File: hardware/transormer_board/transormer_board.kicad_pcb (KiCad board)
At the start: 2 copper layers, 25 x 45 mm, 8 parts, among them J1 orange, J2 black, J3 PE, J4 Conn_02x04_Top_Bottom, J5 red, J6 grey

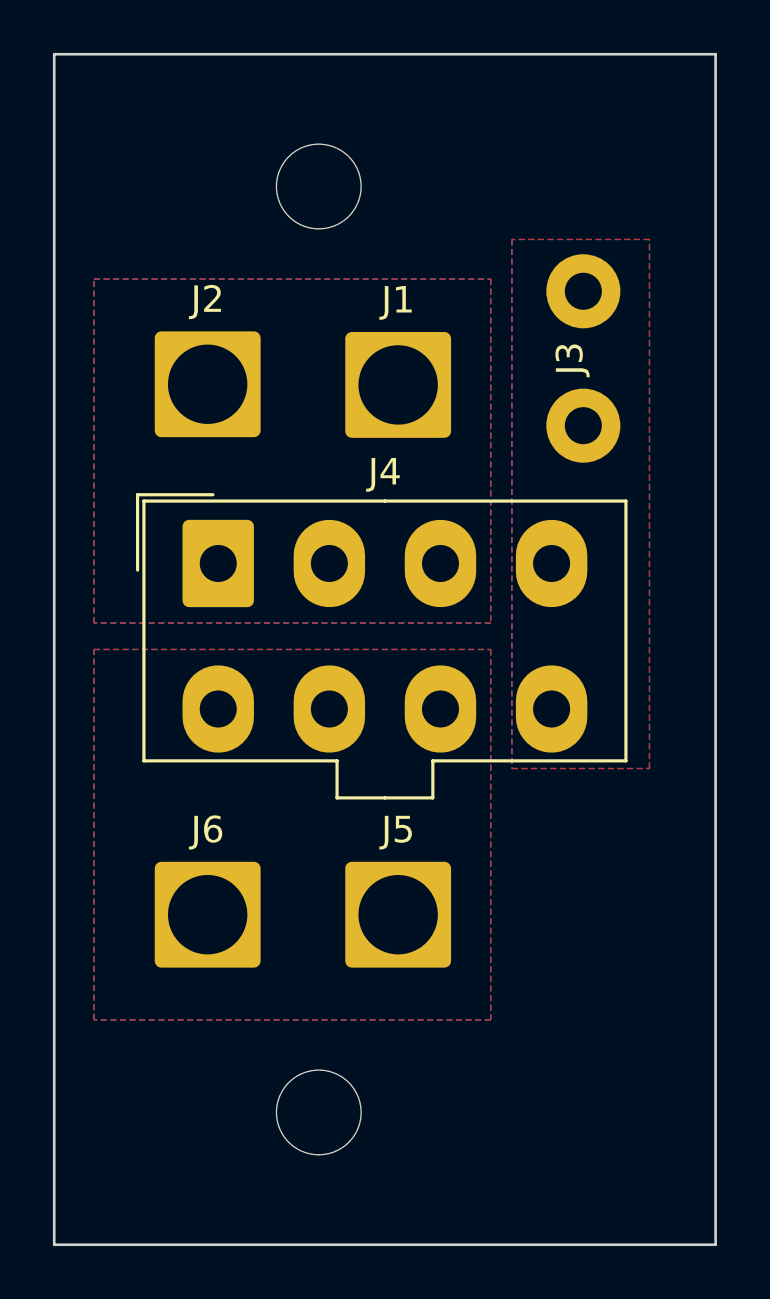
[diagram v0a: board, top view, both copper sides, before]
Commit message: update some shit
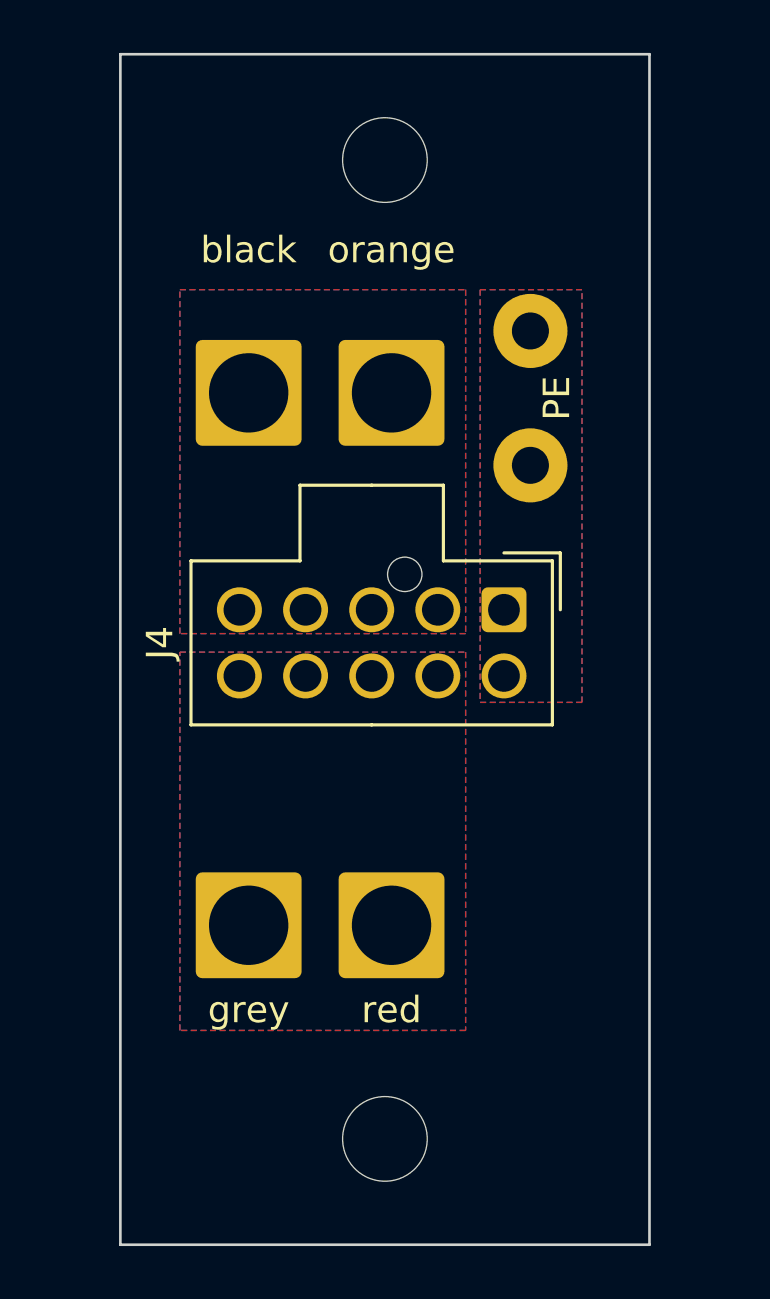
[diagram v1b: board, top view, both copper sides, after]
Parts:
- removed the REF** at (160.0, 121.0)
- removed the REF** at (160.0, 86.0)
- added REF**: MountingHole_3.2mm_M3, MountingHole:MountingHole_3.2mm_M3, F.Cu at (162.5, 122.0)
- added REF**: MountingHole_3.2mm_M3, MountingHole:MountingHole_3.2mm_M3, F.Cu at (162.5, 85.0)
- J4: footprint Connector_Molex:Molex_Mini-Fit_Jr_5566-08A_2x04_P4.20mm_Vertical -> Connector_Molex:Molex_Nano-Fit_105310-xx10_2x05_P2.50mm_Vertical
- moved J4 10.9 mm to (167.0, 102.0), turned to -90 degrees
- moved J3 2.50 mm to (168.0, 94.0)
- moved J6 1.60 mm to (157.3, 113.9)
- moved J2 1.58 mm to (157.3, 93.8)
- moved J5 0.47 mm to (162.8, 113.9)
- moved J1 0.39 mm to (162.8, 93.8)
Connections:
- J4 pad 1: Net-(J1-Pin_1) -> Net-(J3-Pin_1)
- J4 pad 4: Net-(J3-Pin_1) -> Net-(J1-Pin_1)
- J4 pad 5: Net-(J4-Pin_5) -> Net-(J1-Pin_1)
- J4 pad 6: Net-(J4-Pin_5) -> Net-(J3-Pin_1)
- J4 pad 7: Net-(J4-Pin_5) -> Net-(J4-Pin_10)
- J4 pad 8: Net-(J3-Pin_1) -> Net-(J4-Pin_10)
- J5 pad 1: Net-(J4-Pin_5) -> Net-(J4-Pin_10)
- J6 pad 1: Net-(J4-Pin_5) -> Net-(J4-Pin_10)
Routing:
- added copper zone on B.Cu, net Net-(J4-Pin_10)
- added copper zone on F.Cu, net Net-(J4-Pin_10)
- removed copper zone on B.Cu, net Net-(J4-Pin_5)
- removed copper zone on F.Cu, net Net-(J4-Pin_5)
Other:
- board size 25 x 45 mm -> 20 x 45 mm

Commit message: save work
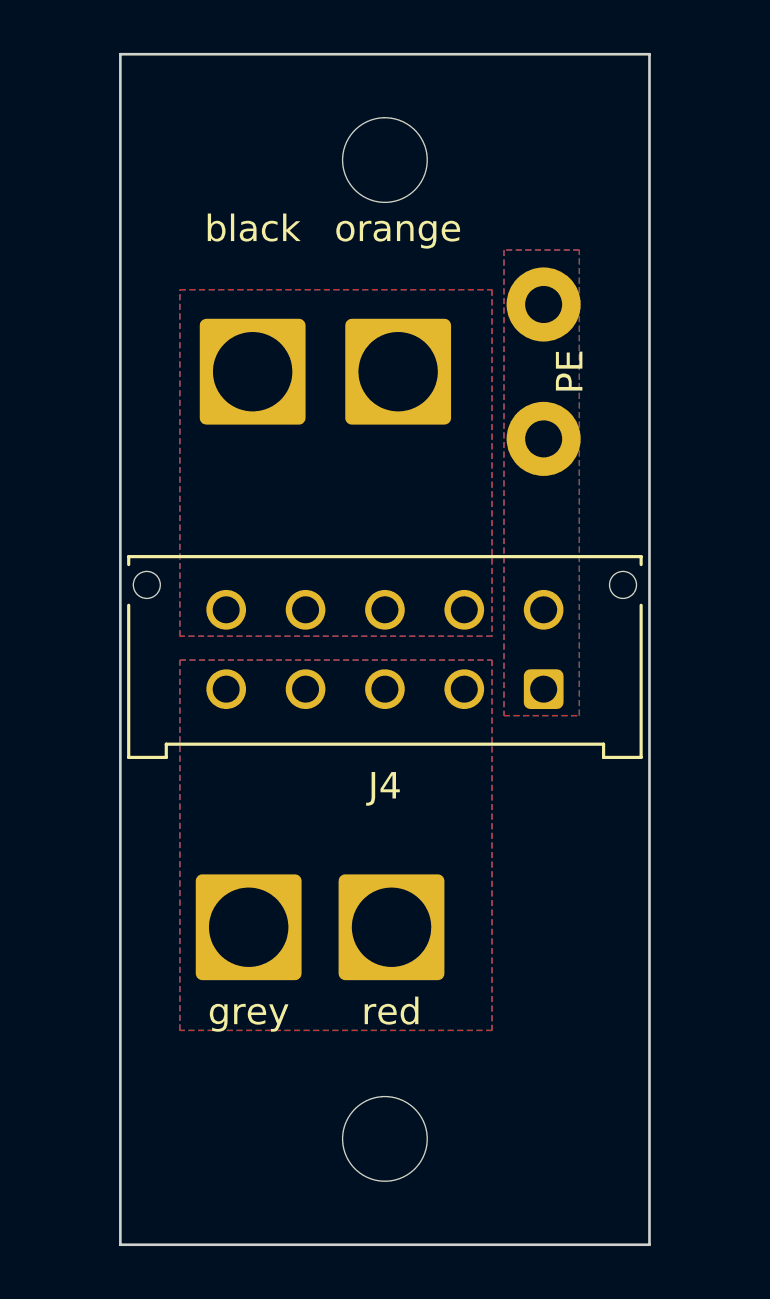
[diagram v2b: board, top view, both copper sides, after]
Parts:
- J4: footprint Connector_Molex:Molex_Nano-Fit_105310-xx10_2x05_P2.50mm_Vertical -> Connector_Molex:Molex_Micro-Fit_3.0_43045-1012_2x05_P3.00mm_Vertical
- moved J4 3.35 mm to (168.5, 105.0), turned to 180 degrees
- moved J3 1.12 mm to (168.5, 93.0)
- moved J1 0.84 mm to (163.0, 93.0)
- moved J2 0.81 mm to (157.5, 93.0)
- moved J5 0.08 mm to (162.8, 114.0)
- moved J6 0.08 mm to (157.3, 114.0)
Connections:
- J4 pad 10: Net-(J4-Pin_10) -> Net-(J1-Pin_1)
- J4 pad 2: Net-(J1-Pin_1) -> Net-(J4-Pin_2)
- J4 pad 3: Net-(J1-Pin_1) -> Net-(J4-Pin_2)
- J4 pad 4: Net-(J1-Pin_1) -> Net-(J4-Pin_2)
- J4 pad 5: Net-(J1-Pin_1) -> Net-(J4-Pin_2)
- J4 pad 7: Net-(J4-Pin_10) -> Net-(J1-Pin_1)
- J4 pad 8: Net-(J4-Pin_10) -> Net-(J1-Pin_1)
- J4 pad 9: Net-(J4-Pin_10) -> Net-(J1-Pin_1)
- J5 pad 1: Net-(J4-Pin_10) -> Net-(J4-Pin_2)
- J6 pad 1: Net-(J4-Pin_10) -> Net-(J4-Pin_2)
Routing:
- added copper zone on B.Cu, net Net-(J4-Pin_2)
- added copper zone on F.Cu, net Net-(J4-Pin_2)
- removed copper zone on B.Cu, net Net-(J4-Pin_10)
- removed copper zone on F.Cu, net Net-(J4-Pin_10)
